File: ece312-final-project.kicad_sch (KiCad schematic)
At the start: 4 parts, among them U1 ATmega328-P, Y1 32.768KHz Crystal

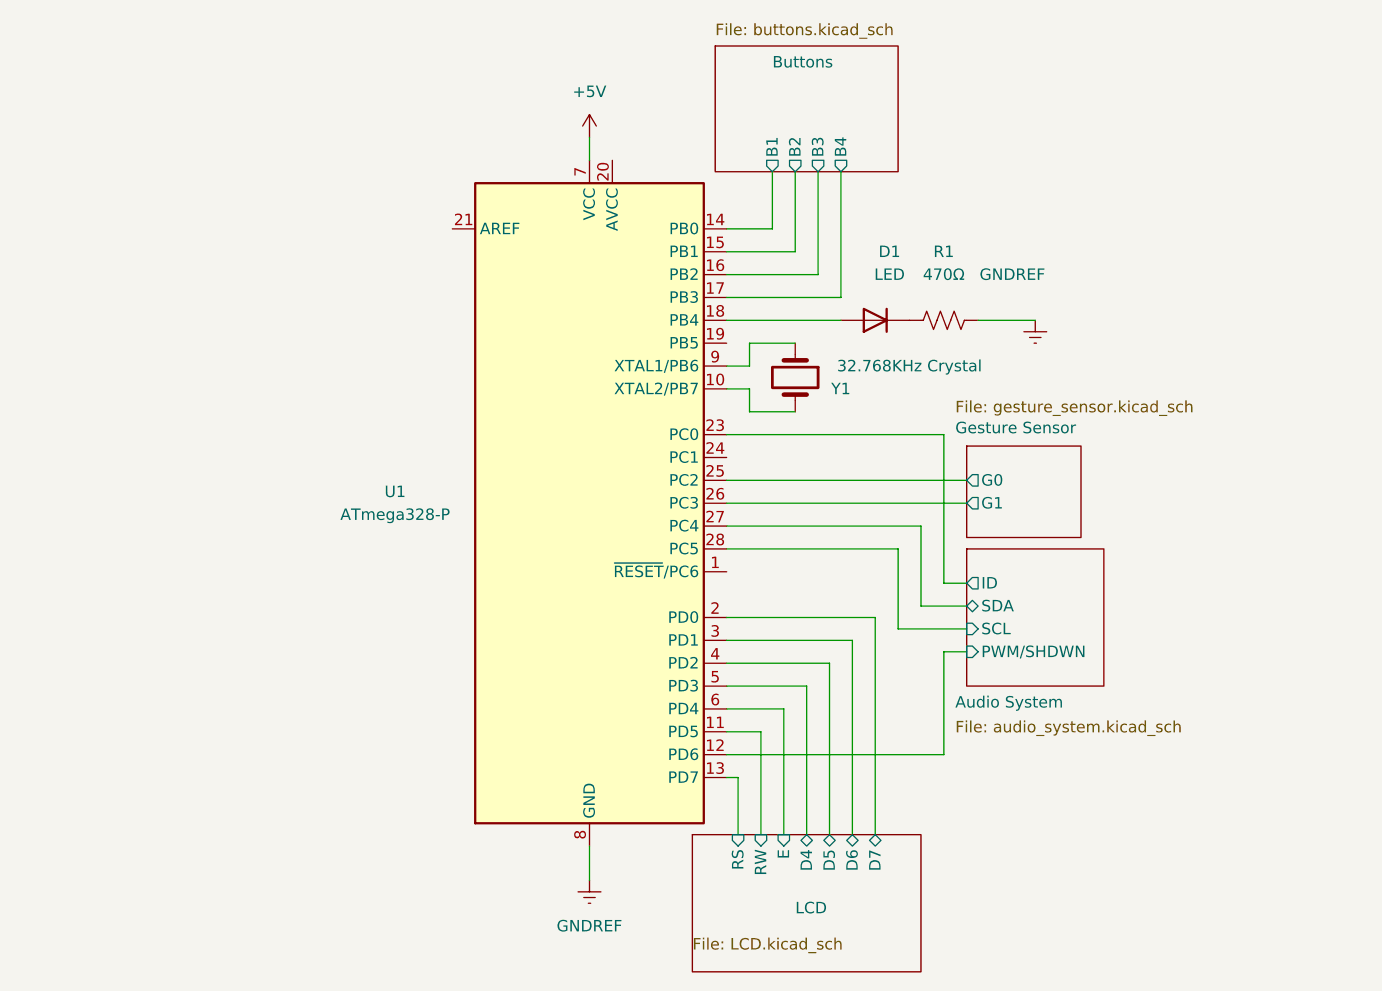
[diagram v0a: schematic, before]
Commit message: Finalized Schematic
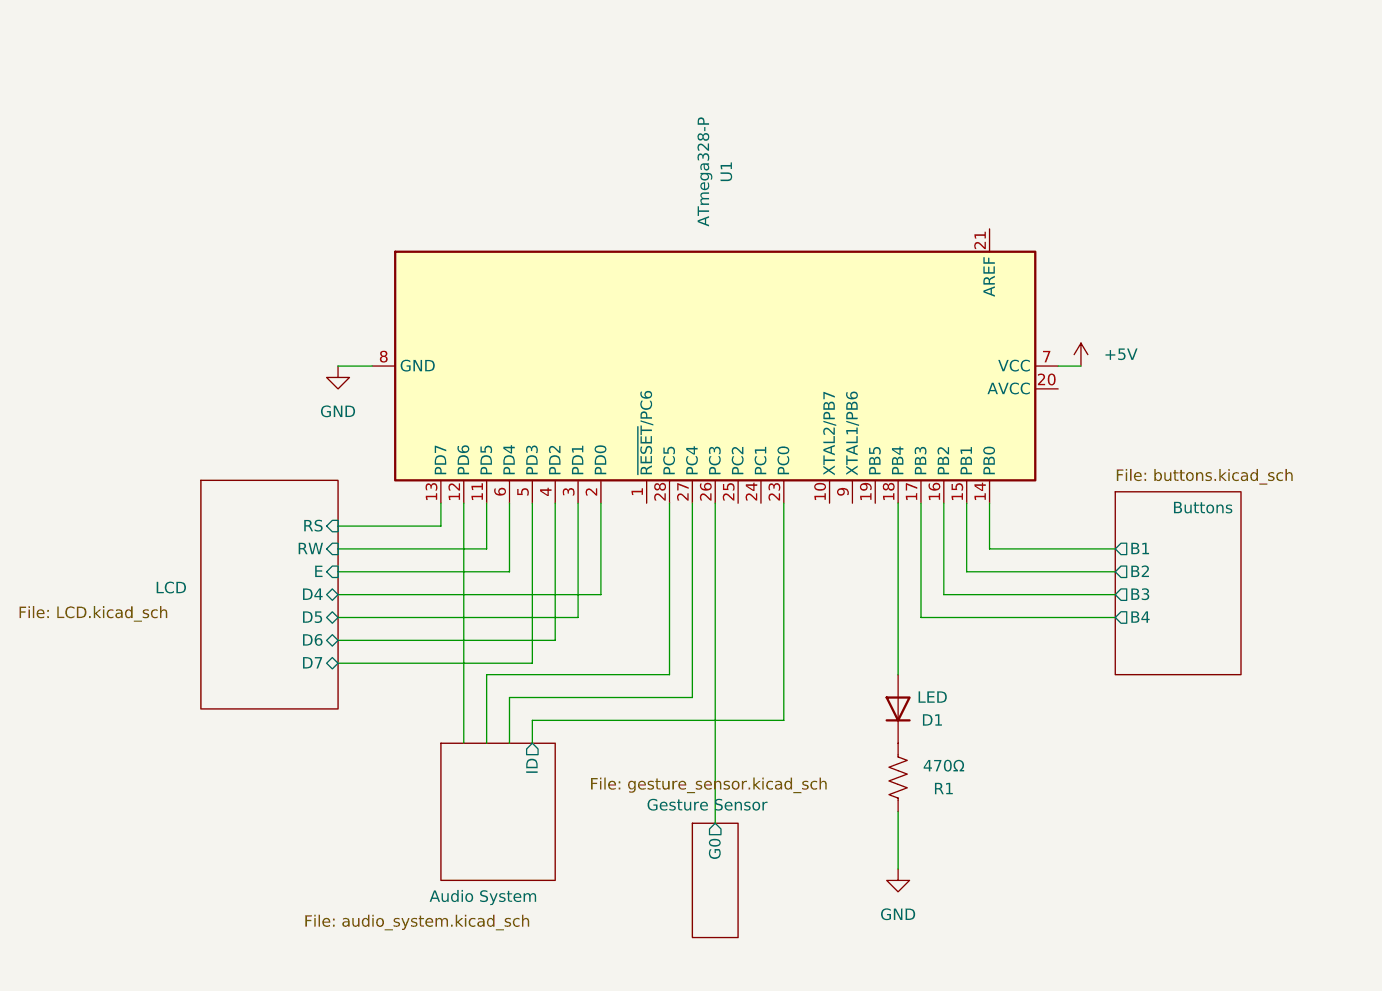
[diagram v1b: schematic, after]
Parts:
- removed Y1: 32.768KHz Crystal, symbol Device:Crystal
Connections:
- net Gesture Sensor/G1 is gone; now on net Gesture Sensor/G0: U1.26 (PC3)
- net Gesture Sensor/G0: no longer U1.25 (PC2)
- net LCD/D4: now also U1.2 (PD0); no longer U1.5 (PD3)
- net LCD/D5: now also U1.3 (PD1); no longer U1.4 (PD2)
- net LCD/D6: now also U1.4 (PD2); no longer U1.3 (PD1)
- net LCD/D7: now also U1.5 (PD3); no longer U1.2 (PD0)
- net Audio System/PWM/SHDWN: no longer names the net of U1.12 (PD6)
- net Audio System/SCL: no longer names the net of U1.28 (PC5)
- net Audio System/SDA: no longer names the net of U1.27 (PC4)
- net GNDREF renamed GND
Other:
- sheet Audio System ports: added none; removed PWM/SHDWN, SCL, SDA
- sheet Gesture Sensor ports: added none; removed G1
- moved on the sheet: D1, R1, U1
